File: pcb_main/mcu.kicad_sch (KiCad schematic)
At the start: 22 parts, among them IC401 OPA277, J401 JST_XH_B2B-XH, Q401 2N7002, Q402 2N7002, U401 REF3240, U402 MCP4725, U403 ATmega328P-A, U404 ADS1115IDGS, U405 MCP4725

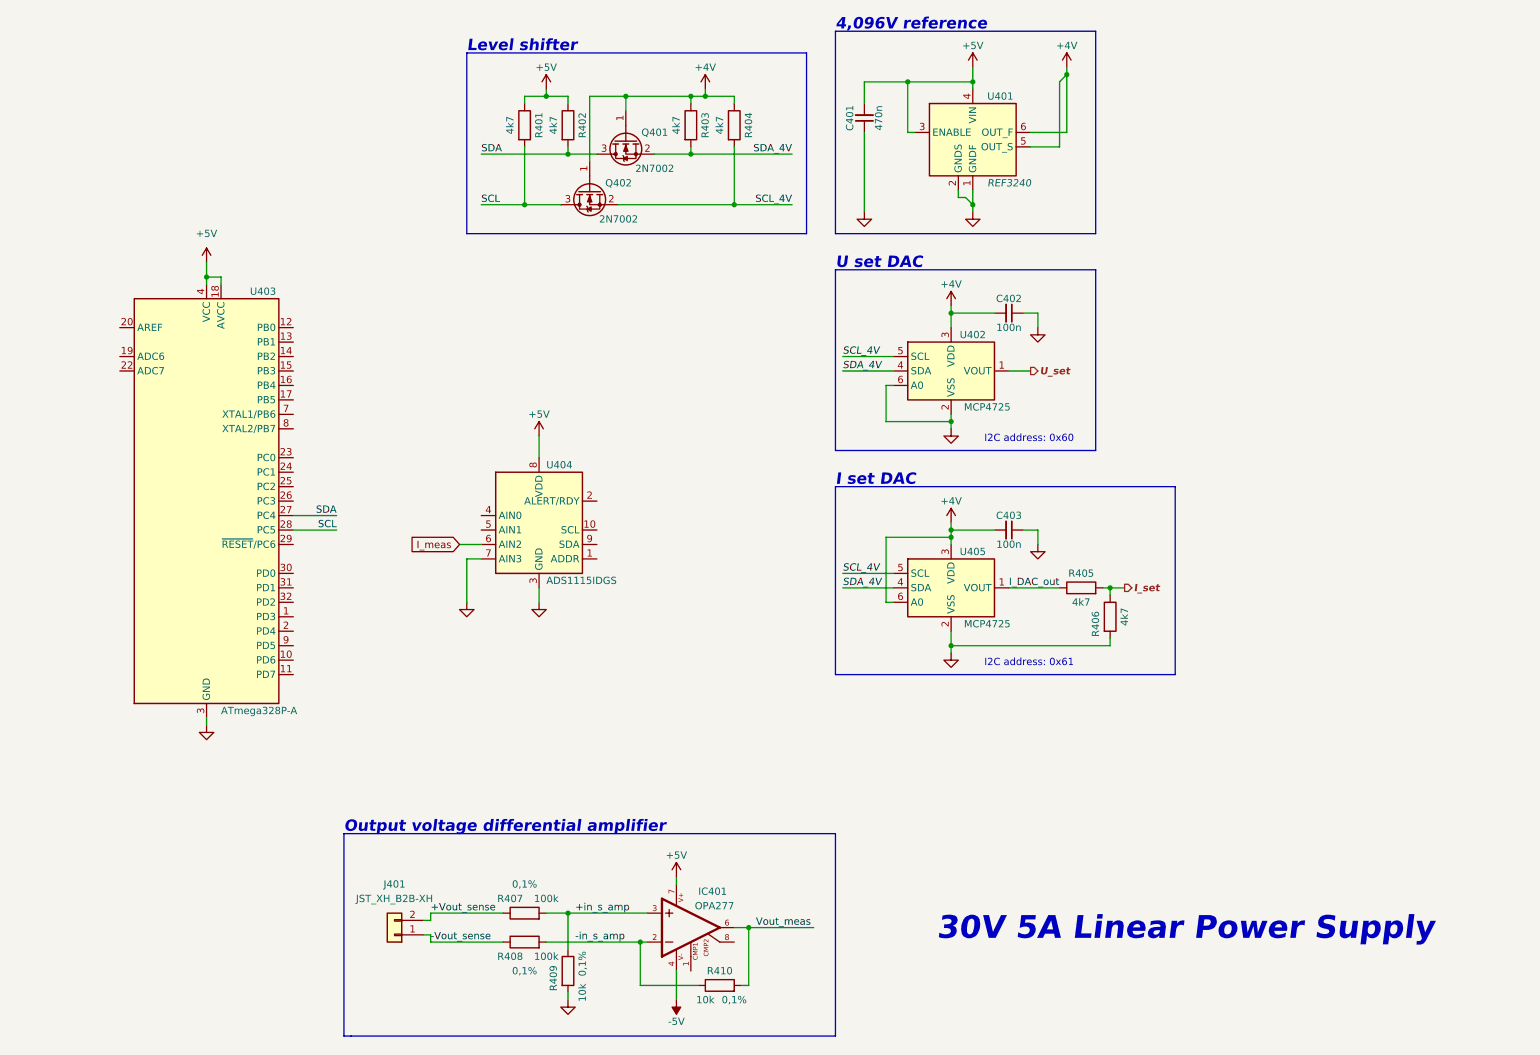
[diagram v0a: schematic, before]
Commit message: most layout done
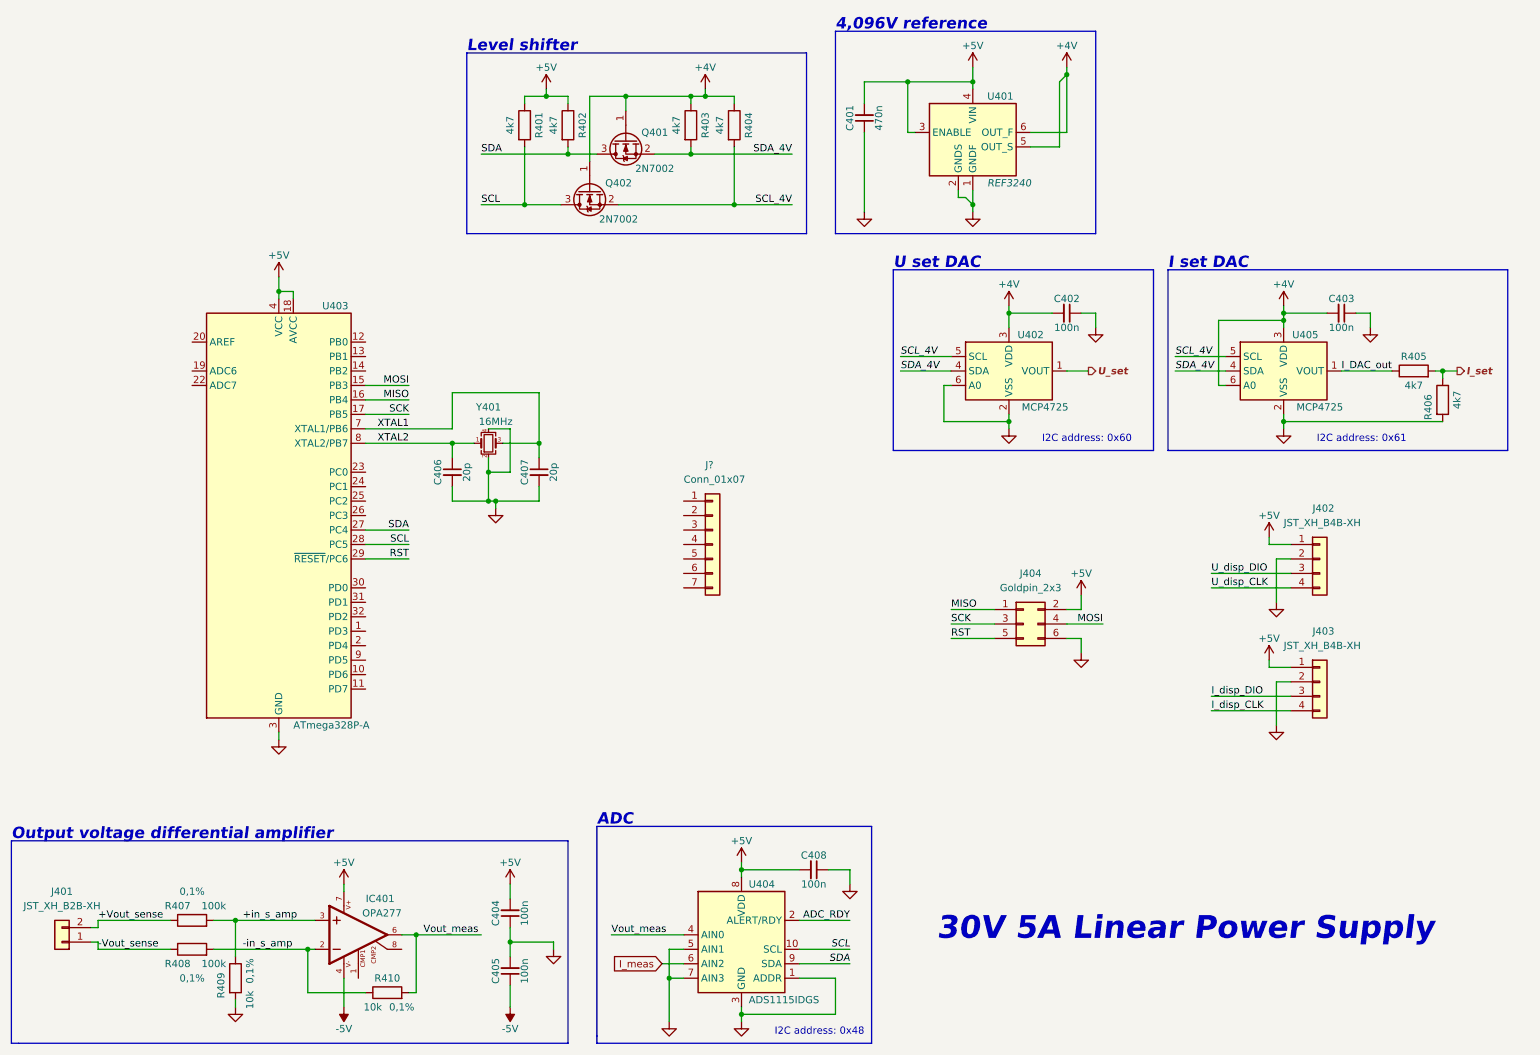
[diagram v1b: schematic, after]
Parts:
- added C404, C405, C408: 100n, Capacitor_SMD:C_0603_1608Metric, symbol Device:C_Small
- added C406, C407: 20p, Capacitor_SMD:C_0603_1608Metric, symbol Device:C_Small
- added J402, J403: JST_XH_B4B-XH, Connector_JST:JST_XH_B4B-XH-A_1x04_P2.50mm_Vertical, symbol Connector_Generic:Conn_01x04
- added J404: Goldpin_2x3, Connector_PinHeader_2.54mm:PinHeader_2x03_P2.54mm_Vertical, symbol Connector_Generic:Conn_02x03_Odd_Even
- added J?: Conn_01x07, Connector_JST:JST_XH_B7B-XH-A_1x07_P2.50mm_Vertical, symbol Connector_Generic:Conn_01x07
- added Y401: 16MHz, Crystal:Crystal_SMD_SeikoEpson_TSX3225-4Pin_3.2x2.5mm, symbol Device:Crystal_GND24_Small
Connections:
- net +5V: now also C404.2, C408.2, J402.1 (Pin_1), J403.1 (Pin_1), J404.2 (Pin_2)
- net -5V: now also C405.1
- net GND: now also U404.1 (ADDR), U404.5 (AIN1), C404.1, C405.2, C406.2, C407.2, C408.1, J402.2 (Pin_2), J403.2 (Pin_2), J404.6 (Pin_6), Y401.2, Y401.4
- net SCL: now also U404.10 (SCL)
- net SDA: now also U404.9 (SDA)
- net Vout_meas: now also U404.4 (AIN0)
- net ADC_RDY: now reaches U404.2 (ALERT/RDY)
- net MOSI: now reaches U403.15 (PB3)
- net MOSI: now also J404.4 (Pin_4)
- net MISO: now reaches U403.16 (PB4)
- net MISO: now also J404.1 (Pin_1)
- net SCK: now reaches U403.17 (PB5)
- net SCK: now also J404.3 (Pin_3)
- net RST: now reaches U403.29 (~{RESET}/PC6)
- net RST: now also J404.5 (Pin_5)
- net XTAL1: now reaches U403.7 (XTAL1/PB6)
- net XTAL1: now also C407.1, Y401.3
- net XTAL2: now reaches U403.8 (XTAL2/PB7)
- net XTAL2: now also C406.1, Y401.1
- new net I_disp_CLK: J403.4 (Pin_4)
- new net I_disp_DIO: J403.3 (Pin_3)
- new net U_disp_CLK: J402.4 (Pin_4)
- new net U_disp_DIO: J402.3 (Pin_3)
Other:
- note added: "ADC"
- note added: "I2C address: 0x48"
- moved on the sheet: C402, C403, IC401, J401, R405, R406, R407, R408, R409, R410, U402, U403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
